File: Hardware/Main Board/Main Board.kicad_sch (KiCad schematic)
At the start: 15 parts, among them J1 Micro_SD_Card_Det1, SW1 SW_SPST, U1 ESP32-S3-WROOM-2

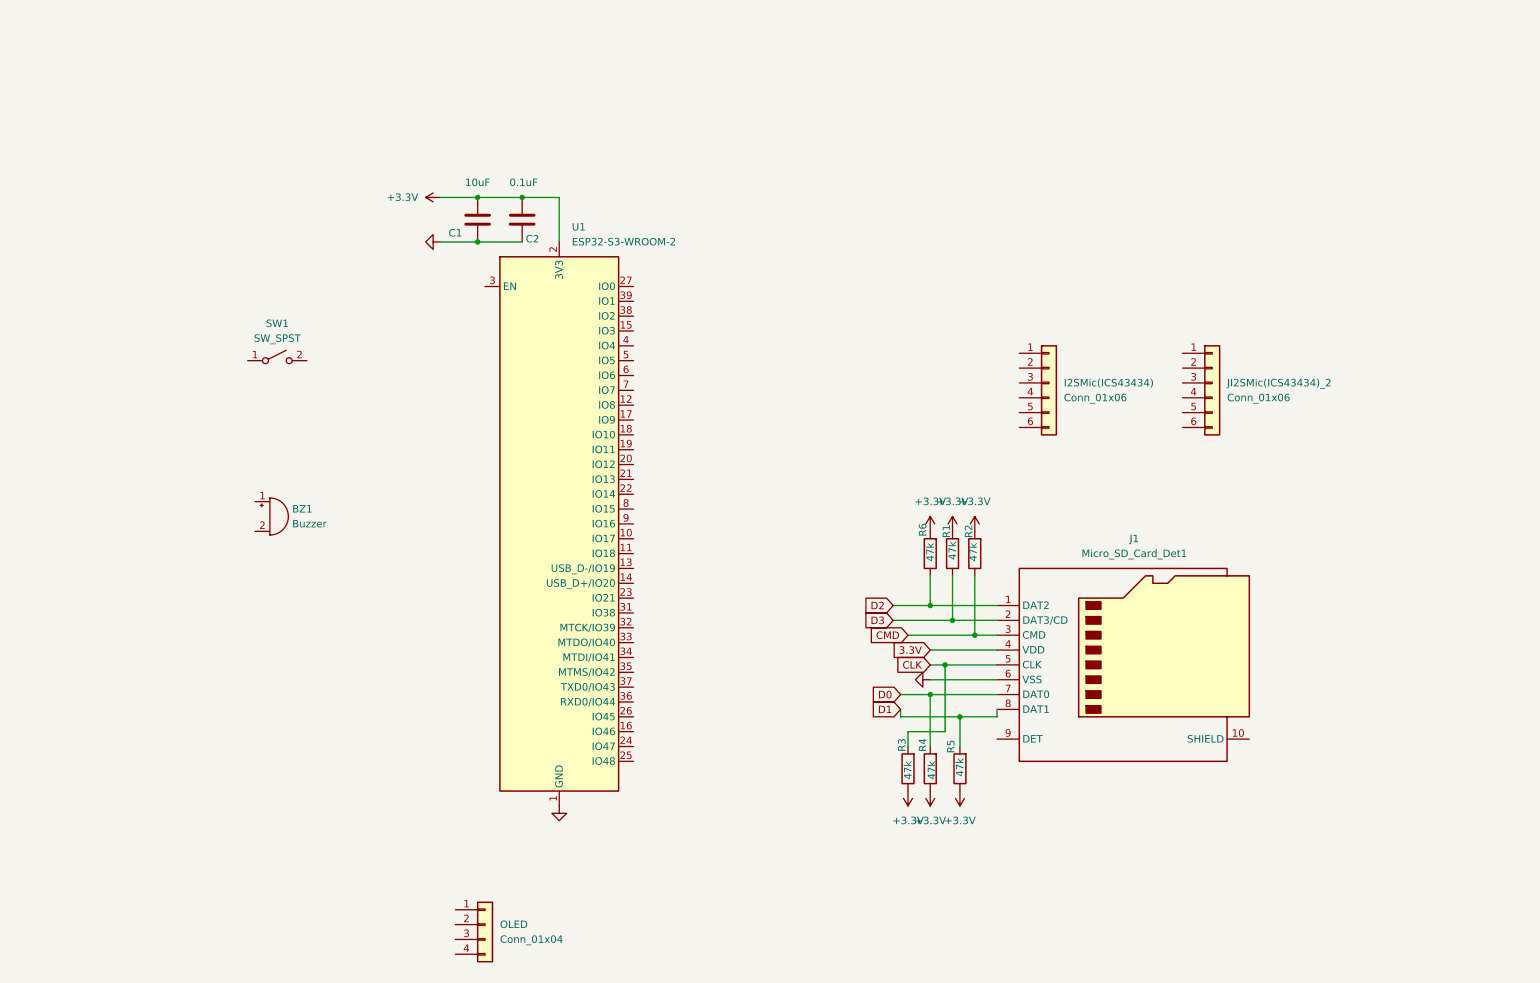
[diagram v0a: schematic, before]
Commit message: schematics for oled and mics
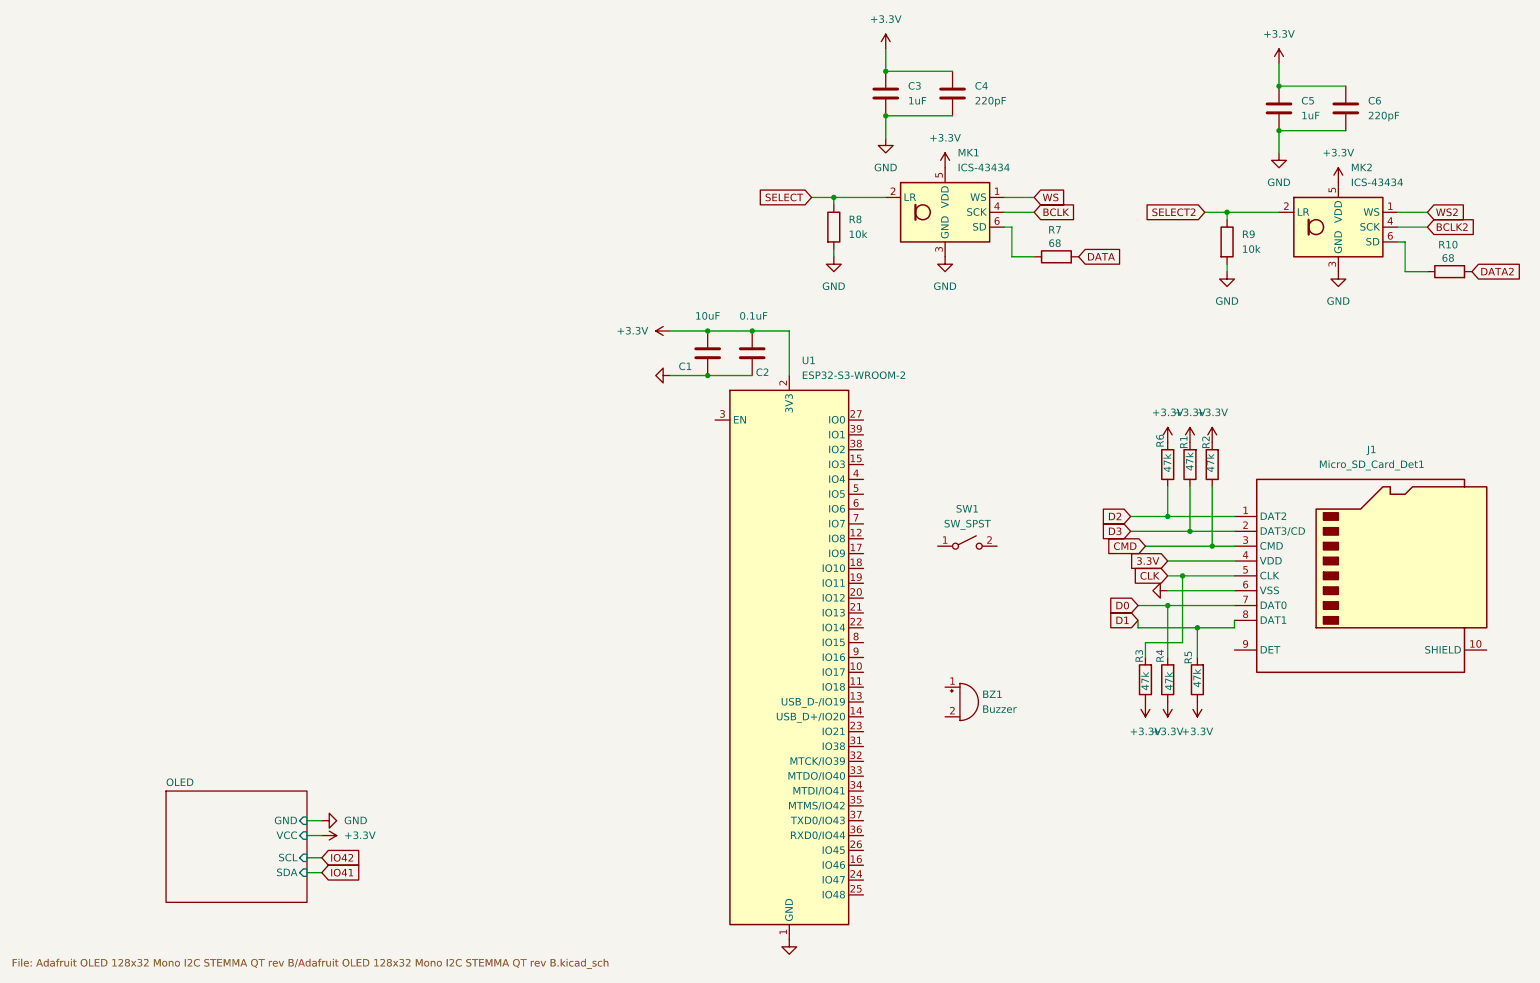
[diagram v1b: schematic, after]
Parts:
- removed I2SMic(ICS43434), JI2SMic(ICS43434)_2: Conn_01x06, symbol Connector_Generic:Conn_01x06
- removed OLED: Conn_01x04, symbol Connector_Generic:Conn_01x04
- added C3, C5: 1uF, symbol Device:C
- added C4, C6: 220pF, symbol Device:C
- added MK1, MK2: ICS-43434, Sensor_Audio:InvenSense_ICS-43434-6_3.5x2.65mm, symbol Sensor_Audio:ICS-43434
- added R10, R7: 68, symbol Device:R
- added R8, R9: 10k, symbol Device:R
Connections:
- net +3.3V: now also C3.1, C4.1, C5.1, C6.1, MK1.5 (VDD), MK2.5 (VDD)
- net GND: now also C3.2, C4.2, C5.2, C6.2, MK1.3 (GND), MK2.3 (GND), R8.2, R9.2
- new net: MK2.6 (SD), R10.1
- new net: MK1.6 (SD), R7.1
- new net BCLK: MK1.4 (SCK)
- new net BCLK2: MK2.4 (SCK)
- new net DATA: R7.2
- new net DATA2: R10.2
- new net SELECT: MK1.2 (LR), R8.1
- new net SELECT2: MK2.2 (LR), R9.1
- new net WS: MK1.1 (WS)
- new net WS2: MK2.1 (WS)
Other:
- added sheet OLED (Adafruit OLED 128x32 Mono I2C STEMMA QT rev B/Adafruit OLED 128x32 Mono I2C STEMMA QT rev B.kicad_sch)
- moved on the sheet: BZ1, C1, C2, J1, R1, R2, R3, R4, R5, R6, SW1, U1
